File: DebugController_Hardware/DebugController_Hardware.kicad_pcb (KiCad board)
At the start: 2 copper layers, 88 parts, among them SW1 SW_Push, SW10 SW_Push, SW11 SW_Push, SW12 SW_Push, SW13 SW_Push, SW14 SW_Push, SW15 SW_Push, SW16 SW_Push, SW17 SW_Push, SW18 SW_Push, SW19 SW_Push, SW2 SW_Push, SW20 SW_Push, SW21 SW_Push, SW22 SW_Push, SW23 SW_Push, SW3 SW_Push, SW4 SW_Push, SW5 SW_Push, SW6 SW_Push, SW7 SW_Push, SW8 SW_Push, SW9 SW_Push, U1 TM4C129E_Launchpad, U2 OKI

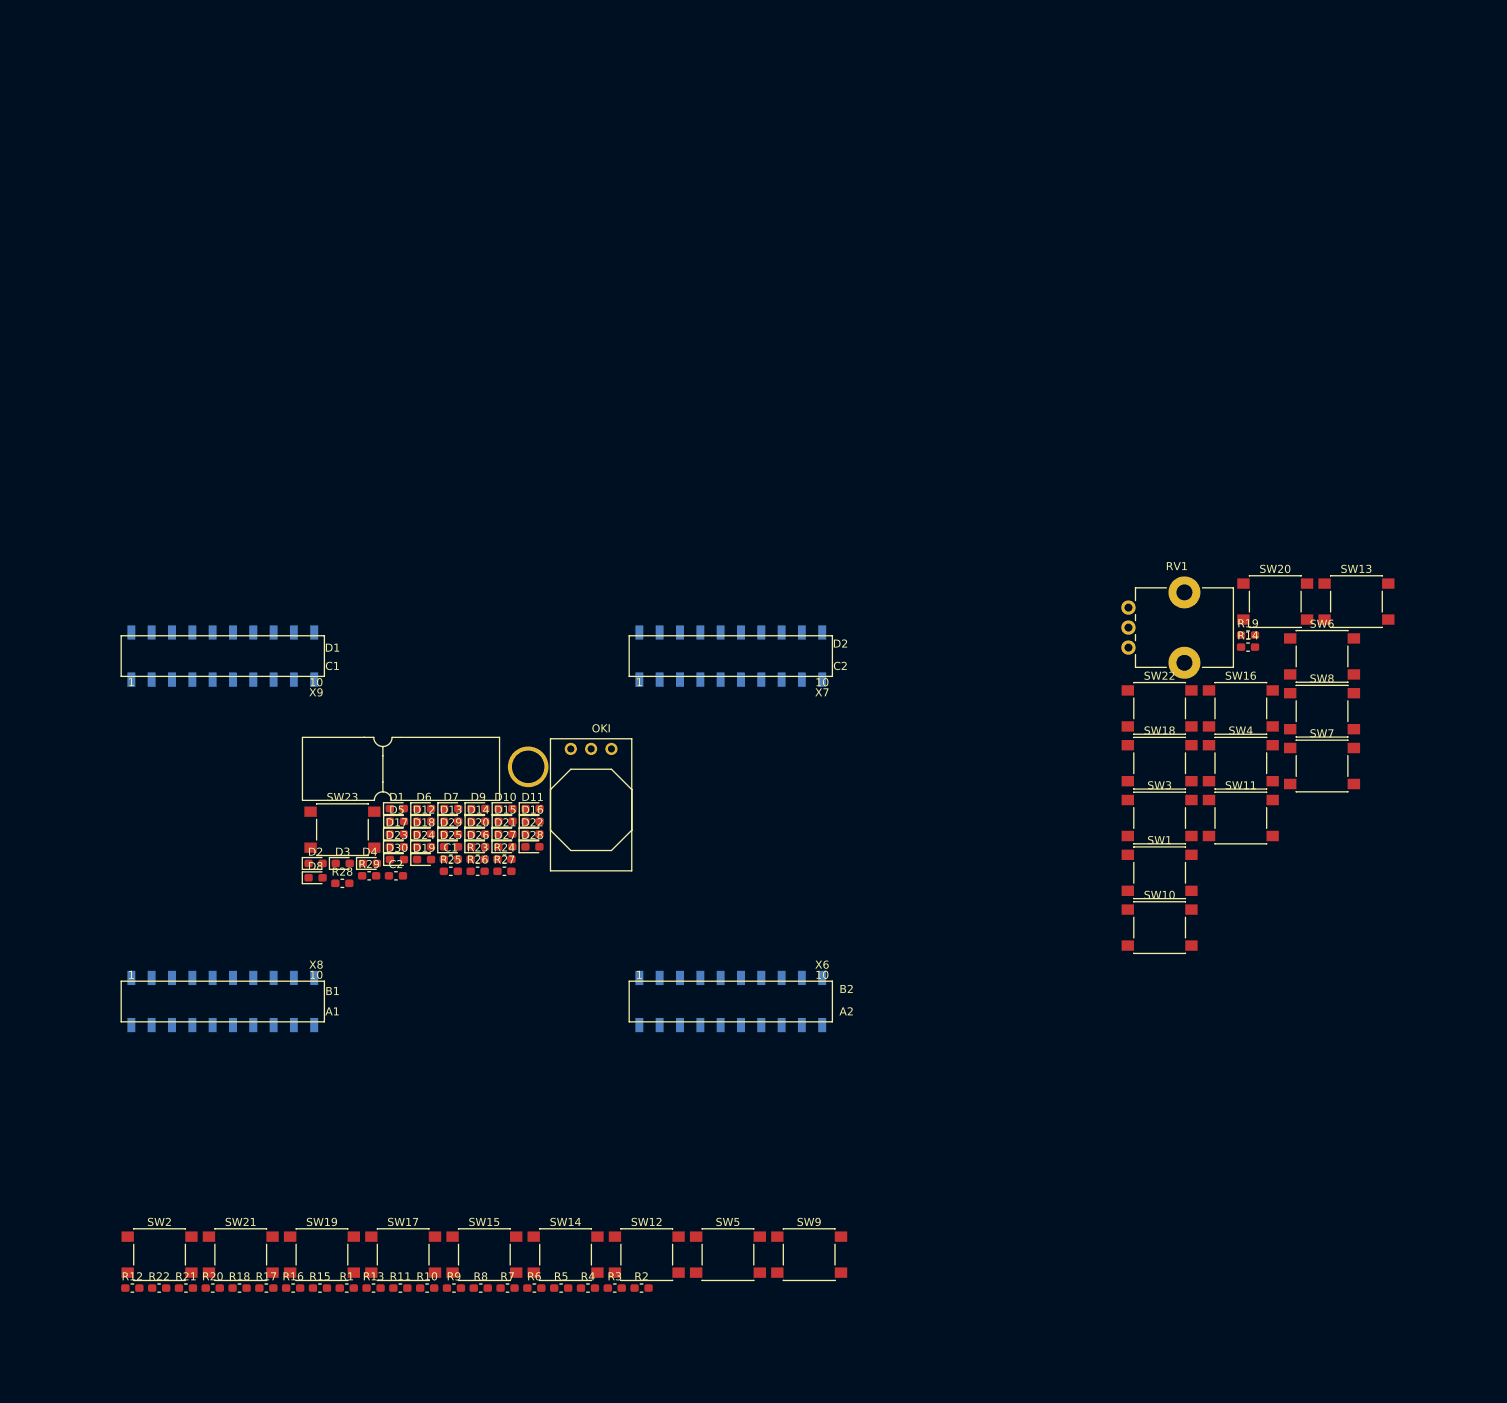
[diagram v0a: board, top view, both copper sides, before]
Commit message: attempted to organize layout
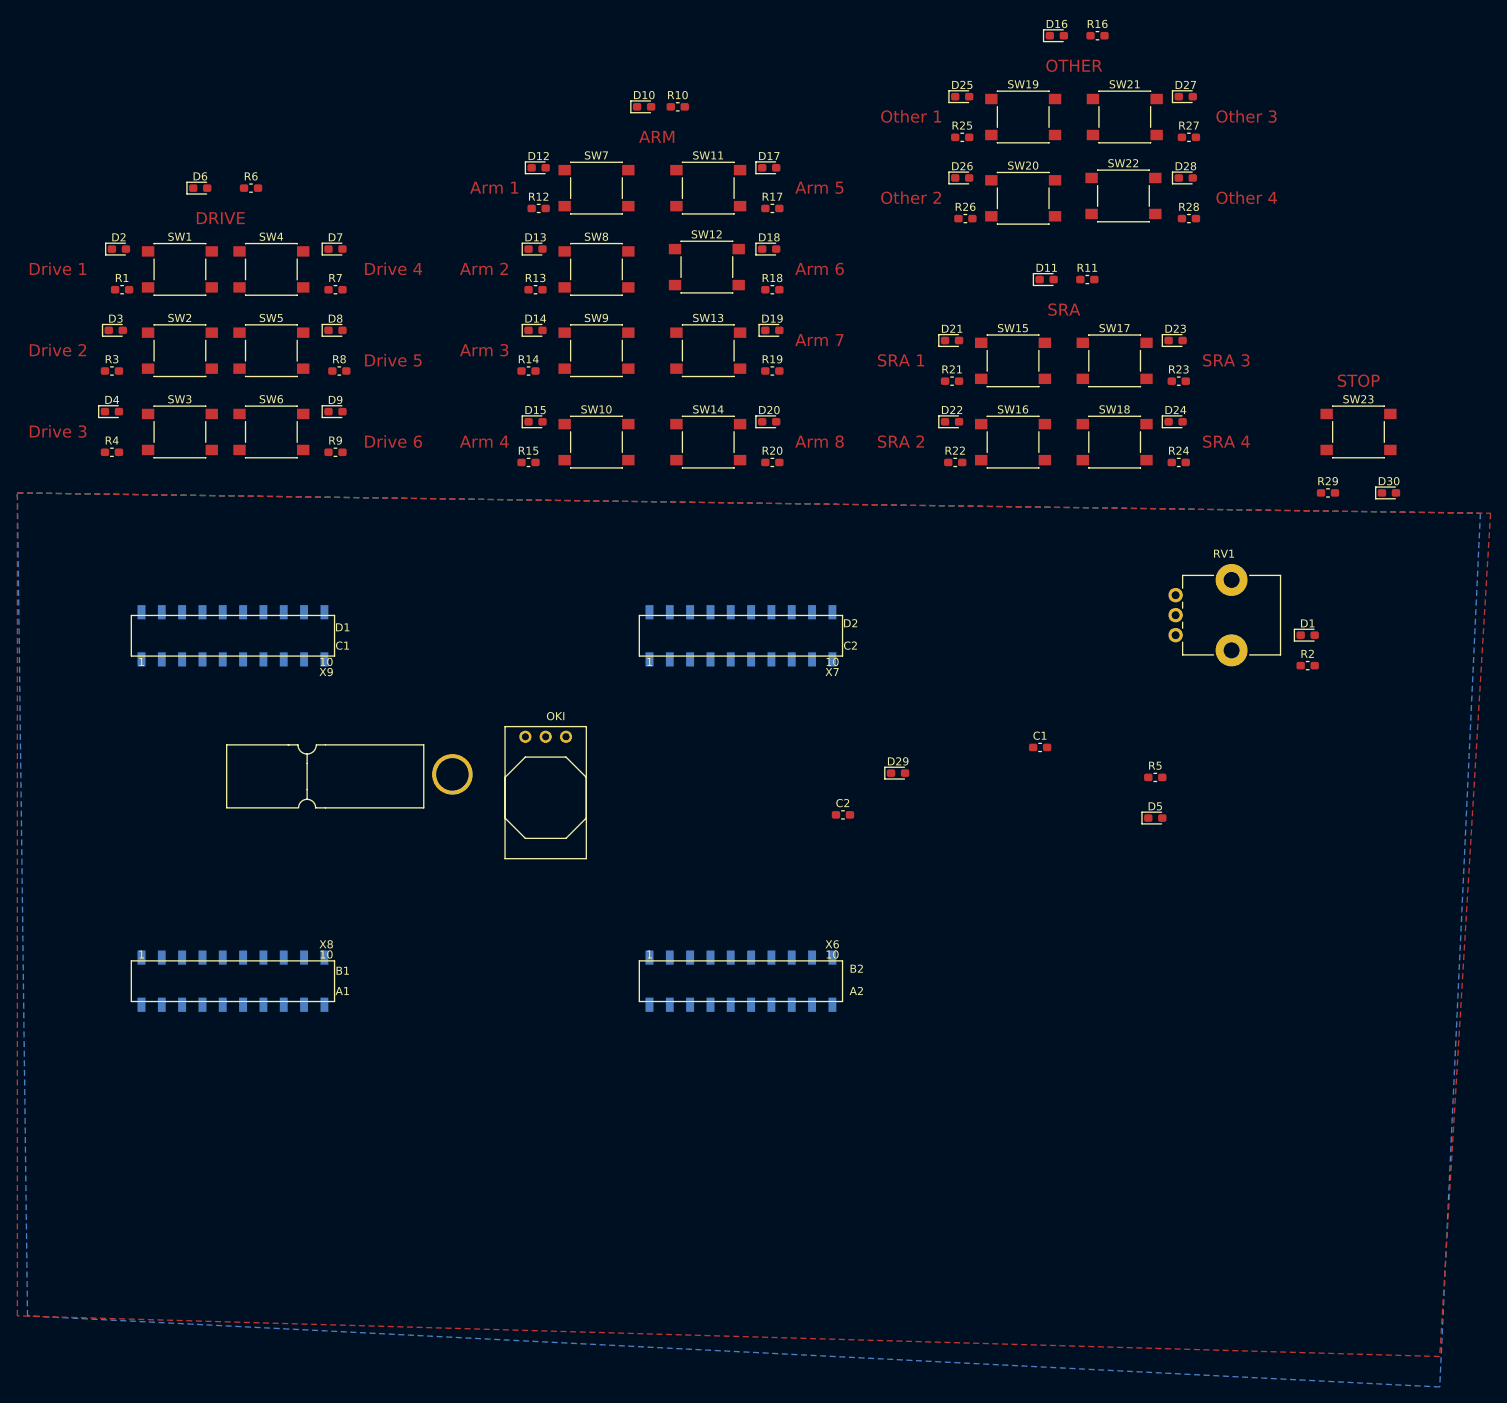
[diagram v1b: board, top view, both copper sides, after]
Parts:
- moved R16 186.1 mm to (137.6, 44.5)
- moved SW21 180.1 mm to (141.0, 54.6)
- moved SW19 167.0 mm to (128.3, 54.6)
- moved R11 152.5 mm to (136.3, 74.9)
- moved R10 150.9 mm to (85.1, 53.3)
- moved R17 149.0 mm to (96.9, 66.0)
- moved R21 148.4 mm to (119.4, 87.6)
- moved R12 144.2 mm to (67.7, 66.0)
- moved SW1 143.8 mm to (22.9, 73.7)
- moved R22 143.4 mm to (119.8, 97.8)
- moved SW17 142.8 mm to (139.7, 85.1)
- moved R6 142.0 mm to (31.8, 63.5)
- moved R18 141.5 mm to (96.9, 76.2)
- moved SW23 136.4 mm to (170.2, 94.0)
- moved SW4 136.0 mm to (34.3, 73.7)
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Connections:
- D5 pad 1: Net-(D5-Pad1) -> GND
- RV1 pad 3: Net-(D29-Pad2) -> GND
- U1 pad +3V3: Net-(U1-Pad+3V3) -> +3V3
- U1 pad GND: Other_1 -> GND
- U1 pad PA6: Arm_7 -> Arm_6
- U1 pad PB4: Net-(U1-PadPB4) -> Drive_Ind
- U1 pad PB5: Net-(U1-PadPB5) -> Arm_Ind
- U1 pad PC7: Drive_Ind -> Net-(U1-PadPC7)
- U1 pad PD0: Net-(U1-PadPD0) -> Other_2
- U1 pad PD1: Net-(U1-PadPD1) -> Other_1
- U1 pad PD4: Pot_Out -> Net-(U1-PadPD4)
- U1 pad PD5: Net-(U1-PadPD5) -> Pot_Out
- U1 pad PD7: Arm_6 -> Arm_5
- U1 pad PE0: Arm_2 -> Arm_1
- U1 pad PE1: Arm_3 -> Arm_2
- U1 pad PE2: Arm_4 -> Arm_3
- U1 pad PE3: Arm_5 -> Arm_4
- U1 pad PH2: Other_3 -> Net-(U1-PadPH2)
- U1 pad PH3: Other_4 -> Net-(U1-PadPH3)
- U1 pad PK0: Net-(U1-PadPK0) -> SRA_Ind
- U1 pad PK1: Net-(U1-PadPK1) -> Other_Ind
- U1 pad PL4: SRA_Ind -> Net-(U1-PadPL4)
- U1 pad PM3: Other_2 -> Net-(U1-PadPM3)
- U1 pad PM4: Arm_8 -> Arm_7
- U1 pad PM5: Arm_Ind -> Arm_8
- U1 pad PN2: Net-(U1-PadPN2) -> Other_3
- U1 pad PN3: Net-(U1-PadPN3) -> Other_4
- U1 pad Rese: Other_Ind -> Net-(U1-PadRese)
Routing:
- added copper zone on B.Cu, net +3V3
- added copper zone on F.Cu, net GND
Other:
- board text added: "ARM"
- board text added: "Arm 1"
- board text added: "Arm 2"
- board text added: "Arm 3"
- board text added: "Arm 4"
- board text added: "Arm 5"
- board text added: "Arm 6"
- board text added: "Arm 7"
- board text added: "Arm 8"
- board text added: "DRIVE"
- board text added: "Drive 1"
- board text added: "Drive 2"
- board text added: "Drive 3"
- board text added: "Drive 4"
- board text added: "Drive 5"
- board text added: "Drive 6"
- board text added: "OTHER"
- board text added: "Other 1"
- board text added: "Other 2"
- board text added: "Other 3"
- board text added: "Other 4"
- board text added: "SRA"
- board text added: "SRA 1"
- board text added: "SRA 2"
- board text added: "SRA 3"
- board text added: "SRA 4"
- board text added: "STOP"
